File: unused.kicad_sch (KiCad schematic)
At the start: 5 parts, among them U1 74LS139, U2 74LS06, U3 NE556

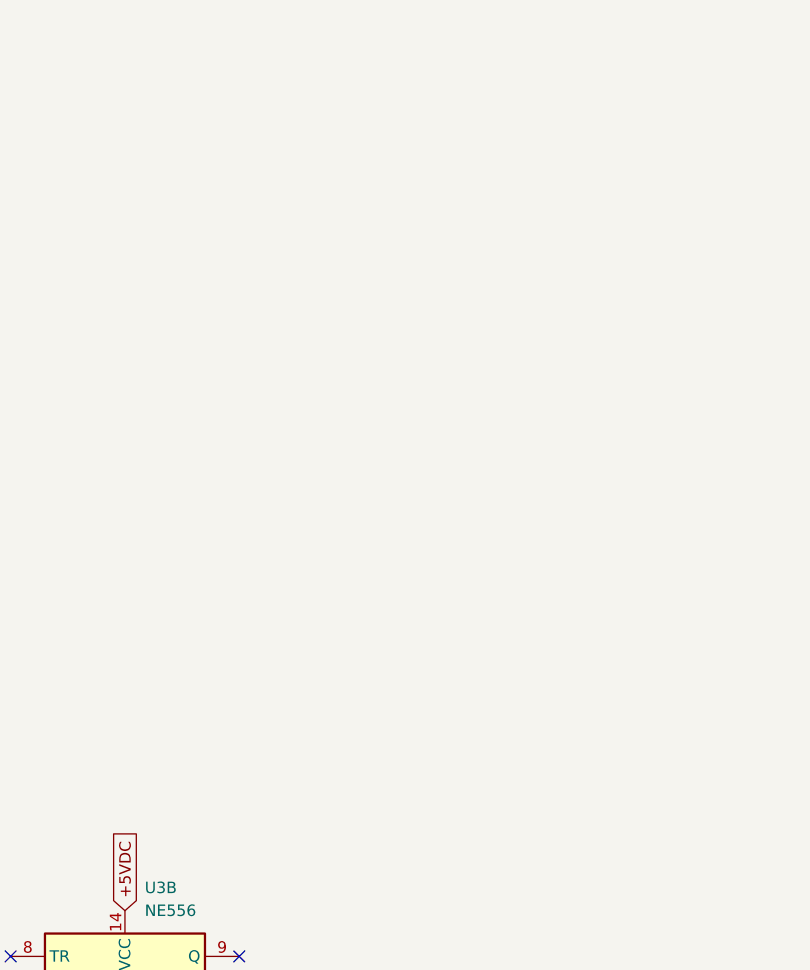
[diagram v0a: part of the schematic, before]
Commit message: Add files via upload
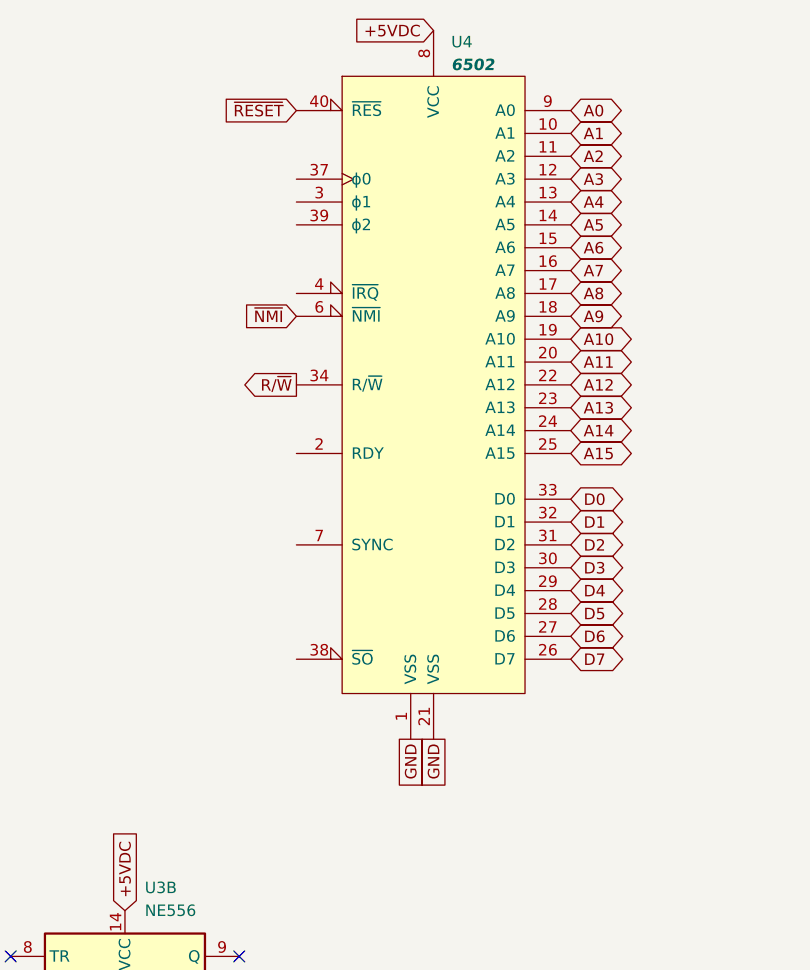
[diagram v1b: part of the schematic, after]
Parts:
- added U4: 6502, Package_DIP:DIP-40_W15.24mm_LongPads, symbol 65xx:6502
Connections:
- net +5VDC: now also U4.8 (VCC)
- net GND: now also U4.1 (VSS), U4.21 (VSS)
- new net A0: U4.9 (A0)
- new net A1: U4.10 (A1)
- new net A10: U4.19 (A10)
- new net A11: U4.20 (A11)
- new net A12: U4.22 (A12)
- new net A13: U4.23 (A13)
- new net A14: U4.24 (A14)
- new net A15: U4.25 (A15)
- new net A2: U4.11 (A2)
- new net A3: U4.12 (A3)
- new net A4: U4.13 (A4)
- new net A5: U4.14 (A5)
- new net A6: U4.15 (A6)
- new net A7: U4.16 (A7)
- new net A8: U4.17 (A8)
- new net A9: U4.18 (A9)
- new net D0: U4.33 (D0)
- new net D1: U4.32 (D1)
- new net D2: U4.31 (D2)
- new net D3: U4.30 (D3)
- new net D4: U4.29 (D4)
- new net D5: U4.28 (D5)
- new net D6: U4.27 (D6)
- new net D7: U4.26 (D7)
- new net R/~{W}: U4.34 (R/~{W})
- new net ~{NMI}: U4.6 (~{NMI})
- new net ~{RESET}: U4.40 (~{RES})
